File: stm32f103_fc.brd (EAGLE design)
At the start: 60.6 x 87.6 mm, 47 parts, among them IC1 STM32F10XCXT6, IC2 LD1117AS33TR, U2 9DoF IMU, Y1 8MHz, Y2 32.768MHz

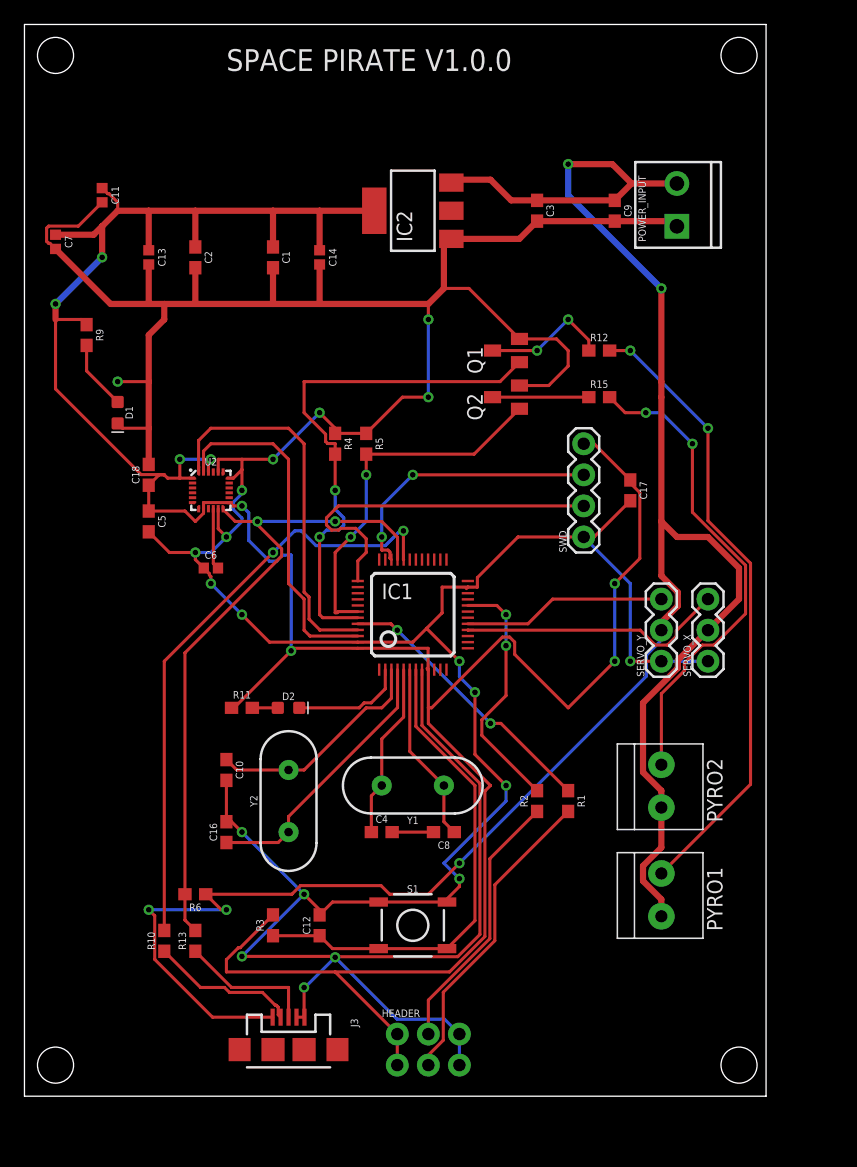
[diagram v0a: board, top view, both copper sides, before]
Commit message: done version 2
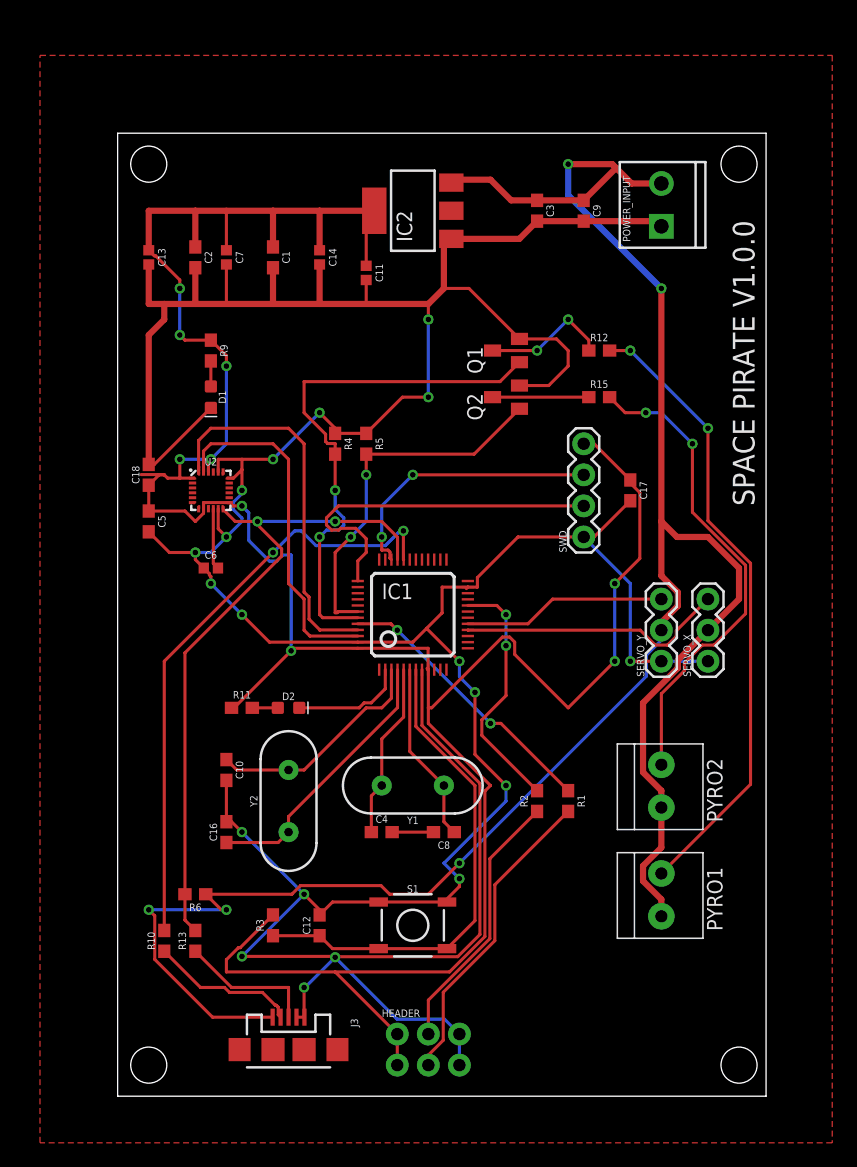
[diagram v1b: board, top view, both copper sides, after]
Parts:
- moved C11 22.5 mm to (39.4, 78.7)
- moved C7 14.0 mm to (27.9, 80.0)
- moved R9 10.2 mm to (26.7, 72.4)
- moved D1 7.73 mm to (26.7, 68.6)
- moved C9 2.54 mm to (57.1, 83.8)
- moved POWER_INPUT 1.27 mm to (63.5, 82.5)
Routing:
- net GND: track 354.0 -> 343.3 mm, vias 20 -> 19
- net VCC3V3: track 232.6 -> 223.8 mm, vias 8 -> 9
- net N$3: track 5.68 -> 2.08 mm
- net 5V: track 182.3 -> 180.3 mm
- added copper zone on layer 1, net GND
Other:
- board size 60.6 x 87.6 mm -> 53 x 78.7 mm
